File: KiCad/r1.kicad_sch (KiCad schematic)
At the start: 73 parts, among them J1 KEYBOARD, J2 VIDEO OUT, J3 ATX-20, J4 DE9_Socket, J5 R1 EXPANSION, Q1 2N4401, SW1 RESET, SW2 CLEAR, U1 6502, U10 74LS245, U11 MAX232, U2 6821, U3 27C64, U4 HM62256BLP, U5 74LS138, U6 74LS00, U7 74LS04, U8 P8X32A-D40, U9 24LC256, X1 1 MHz, X2 5MHz

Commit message: Unzipped and rearranged directories
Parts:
- added C21: 100, Capacitor_THT:CP_Radial_D10.0mm_P5.00mm, symbol Device:C_Polarized
- added C22: 100, Capacitor_THT:CP_Radial_D5.0mm_P2.50mm, symbol Device:C_Polarized
- added S1: ON/OFF, Button_Switch_THT:SW_PUSH_6mm, symbol Switch:SW_DPST
- D1: value LED -> POWER; footprint (none) -> LED_THT:LED_D5.0mm
- JP1, JP2: footprint (none) -> TestPoint:TestPoint_Bridge_Pitch2.54mm_Drill1.0mm
- S3: renamed from SW2; footprint (none) -> Button_Switch_THT:SW_PUSH_6mm
- renumbered SW1 to S2
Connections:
- net -12V: now also J3.12 (-12V), J5.1 (Pin_1), C22.2
- net A0: now also J5.4 (Pin_4), U3.10 (A0), U4.10 (A0)
- net A1: now also J5.24 (Pin_24), U3.9 (A1), U4.9 (A1)
- net A10: now also J5.9 (Pin_9), U3.21 (A10), U4.21 (A10)
- net A11: now also J5.29 (Pin_29), U3.23 (A11), U4.23 (A11)
- net A12: now also J5.10 (Pin_10), U3.2 (A12), U4.2 (A12), U5.1 (A0)
- net A13: now also J5.30 (Pin_30), U4.26 (A13), U5.2 (A1)
- net A14: now also J5.11 (Pin_11), U4.1 (A14), U5.3 (A2)
- net A15: now also J5.31 (Pin_31), U4.20 (~{CS}), U4.22 (~{OE}), U5.6 (E3)
- net A2: now also J5.5 (Pin_5), U3.8 (A2), U4.8 (A2)
- net A3: now also J5.25 (Pin_25), U3.7 (A3), U4.7 (A3)
- net A4: now also J5.6 (Pin_6), U3.6 (A4), U4.6 (A4)
- net A5: now also J5.26 (Pin_26), U3.5 (A5), U4.5 (A5)
- net A6: now also J5.7 (Pin_7), U3.4 (A6), U4.4 (A6)
- net A7: now also J5.27 (Pin_27), U3.3 (A7), U4.3 (A7)
- net A8: now also J5.8 (Pin_8), U3.25 (A8), U4.25 (A8)
- net A9: now also J5.28 (Pin_28), U3.24 (A9), U4.24 (A9)
- net D0: now also J5.33 (Pin_33), U3.11 (D0), U4.11 (Q0)
- net D1: now also J5.15 (Pin_15), U3.12 (D1), U4.12 (Q1)
- net D2: now also J5.34 (Pin_34), U3.13 (D2), U4.13 (Q2)
- net D3: now also J5.16 (Pin_16), U3.15 (D3), U4.15 (Q3)
- net D4: now also J5.35 (Pin_35), U3.16 (D4), U4.16 (Q4)
- net D5: now also J5.17 (Pin_17), U3.17 (D5), U4.17 (Q5)
- net D6: now also J5.36 (Pin_36), U3.18 (D6), U4.18 (Q6)
- net D7: now also J5.18 (Pin_18), U3.19 (D7), U4.19 (Q7)
- net GND: now also C14.2, C15.2, C19.1, C20.2, C8.1, C9.1, D1.2 (A), J3.13 (GND), J3.15 (GND), J3.16 (GND), J3.17 (GND), J3.3 (GND), J3.5 (GND), J3.7 (GND), J4.5, J5.3 (Pin_3), Q1.3 (E), R24.2, U11.15 (GND), U5.4 (E1), U5.5 (E2), U5.8 (GND), V1.2 (GND), V2.2 (GND), C21.2, C22.1, S1.2; no longer C8.2, C9.2
- net IRQ: now also J5.38 (Pin_38)
- net NMI: now also J5.39 (Pin_39)
- net PHI0: now also J5.23 (Pin_23)
- net PHI1: now also J5.14 (Pin_14)
- net PHI2: now also J5.20 (Pin_20), U6.12
- net RDY: now also J5.37 (Pin_37)
- net RESET: now also J5.40 (Pin_40)
- net RX: now also R18.1
- net R/W: now also J5.12 (Pin_12), U6.4, U6.5
- net SYNC: now also J5.19 (Pin_19)
- net TX: now also U11.11 (T1IN)
- net VCC: now also C14.1, C18.2, C20.1, J3.19 (+5V), J3.20 (+5V), J3.4 (+5V), J3.6 (+5V), J5.21 (Pin_21), R20.2, U11.16 (VCC), U3.27 (~{PGM}), U3.28 (VCC), U4.28 (VCC), U5.16 (VCC), V1.3 (VO), V2.1 (IN)
- net VDD: now also C15.1, C8.2, C9.2, R6.1, V2.3 (OUT); no longer C8.1, C9.1, R6.2
- net at J2.1 (In), R17.1: now also R21.1, R23.2; no longer R18.1, R19.1
- net at R18.2: now also U11.12 (R1OUT); no longer U8.18 (P13)
- net at R23.1: now also U8.18 (P13)
- net at R25.1: now also C13.2
- net at R25.2: now also Q1.2 (B), R24.1
- net at U6.6: now also U6.13
- net RST: now reaches JP2.2 (B), S3.2, U8.11 (~{RES})
- net RST: now also Q1.1 (C)
- net at U8.19 (P14): now also R21.2; no longer R19.2
- net at U8.38 (P29), U9.5 (SDA): now also R6.2; no longer R6.1
- net at U4.27 (~{WE}): now also U6.11
- net at U6.10: now also U6.3, U6.9
- net at U6.8: now also U3.20 (~{CE}), U3.22 (~{OE})
- net at C17.1: now also U11.4 (C2+)
- net at C17.2: now also U11.5 (C2-)
- net at C16.1: now also U11.1 (C1+)
- net at C16.2: now also U11.3 (C1-)
- net at R20.1: now also D1.1 (K)
- net at V1.1 (VI): now also C21.1, S1.4
- net at U11.13 (R1IN): now also J4.3
- net at U11.14 (T1OUT): now also J4.2
- net at U11.2 (VS+): now also C18.1
- net at U11.6 (VS-): now also C19.2
- net $D000: now reaches U5.10 (O5)
- net $C000: now reaches U5.11 (O4)
- net $C000: now also J5.22 (Pin_22)
- net $B000: now reaches U5.12 (O3)
- net $B000: now also J5.32 (Pin_32)
- net $A000: now reaches U5.13 (O2)
- net $A000: now also J5.13 (Pin_13)
- net at U5.7 (O7): now also U6.2
- net at U5.9 (O6): now also U6.1
- net at J4.1: now also J4.6
- net at J4.4: now also C13.1
- net 12V: now reaches J3.10 (+12V)
- net 12V: now also J5.2 (Pin_2)
- net at J3.14 (PS_ON#): now also S1.1
- no-connect marks 10 -> 26
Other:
- moved on the sheet: C13, C14, C15, C16, C17, C18, C19, C20, C8, C9, D1, J1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

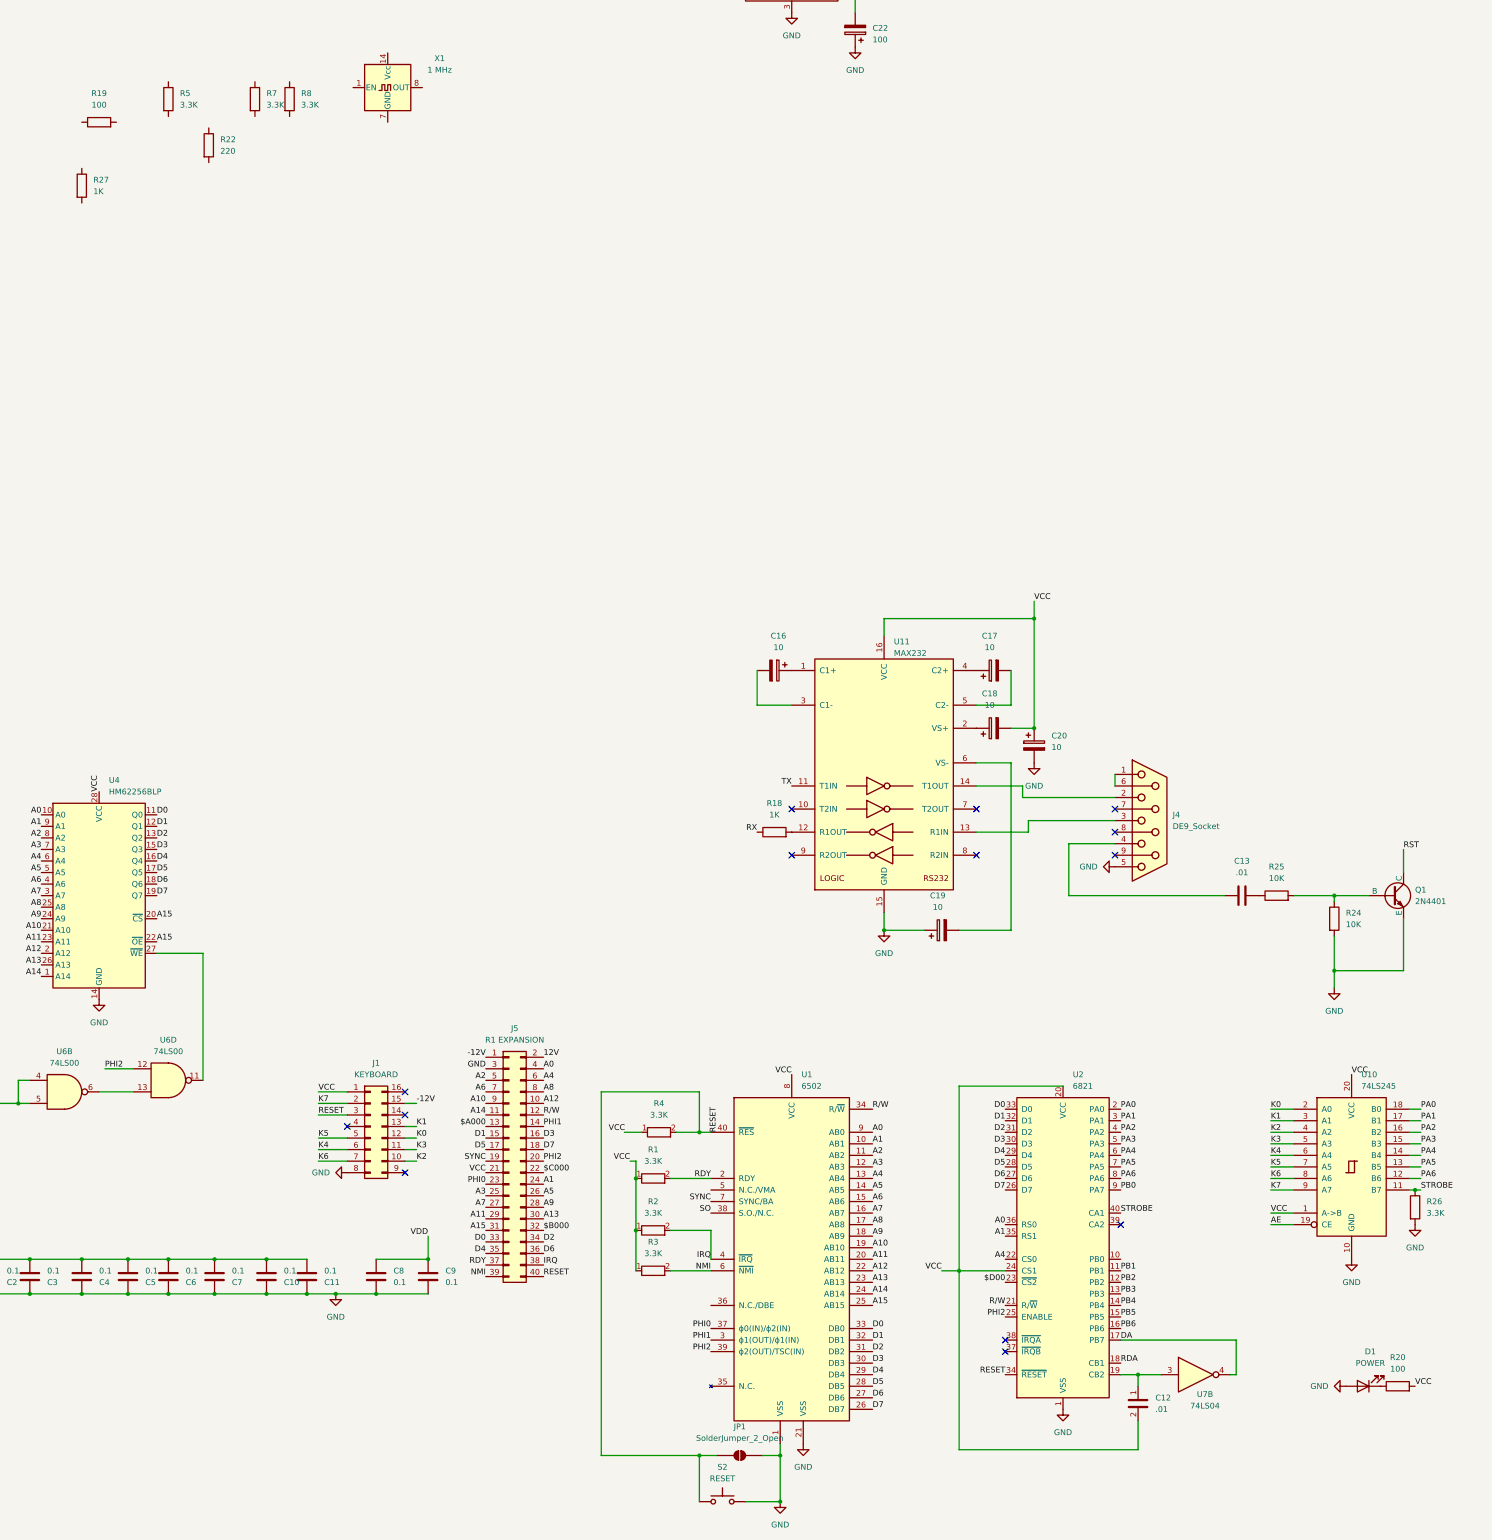
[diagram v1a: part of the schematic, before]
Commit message: R20260909
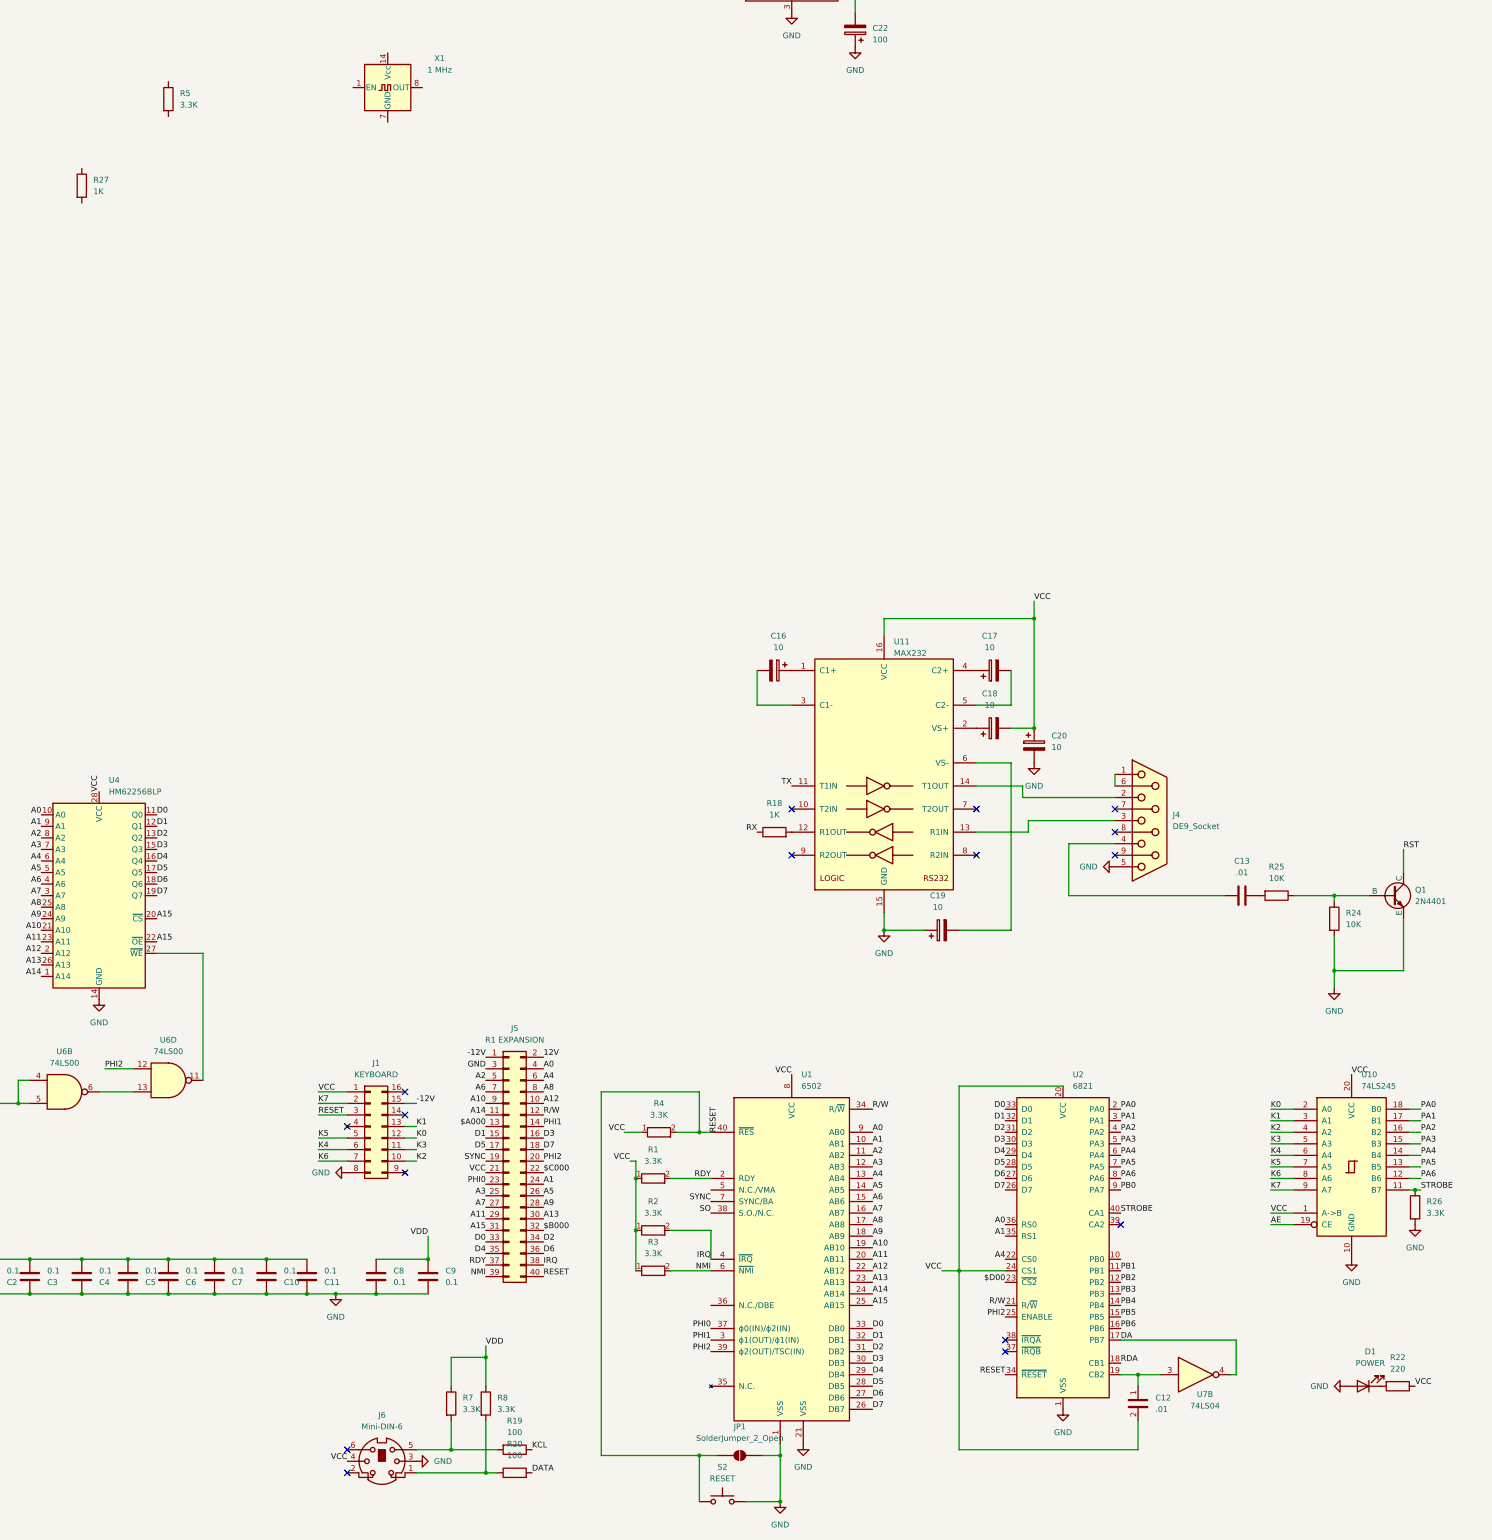
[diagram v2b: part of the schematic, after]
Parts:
- added J6: Mini-DIN-6, symbol Connector:Mini-DIN-6
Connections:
- net GND: now also J6.3
- net KCL: now also R19.1
- net VCC: now also R22.1, J6.4; no longer R20.2
- net VDD: now also R7.1, R8.1
- net at R8.2: now also R20.1, J6.1
- net at R25.1: now also Q1.2 (B), R24.1; no longer C13.2
- net at R19.2: now also R7.2, J6.5
- net at R22.2: now also D1.1 (K)
- new net: C13.2, R25.2
- new net DATA: R20.2
- no-connect marks 26 -> 28
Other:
- moved on the sheet: R19, R20, R22, R25, R7, R8
